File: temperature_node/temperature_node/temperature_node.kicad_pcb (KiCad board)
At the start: 4 copper layers, 21 x 34 mm, 34 parts, among them CN1 UART, J1 USB_C_Receptacle_USB2.0_16P, J2 S2B-PH-K-S, U1 SHT40-AD1B-R3, U2 MCP73831-2-OT, U3 MIC5504-3.3YM5, U4 ESP32-C3-WROOM-02

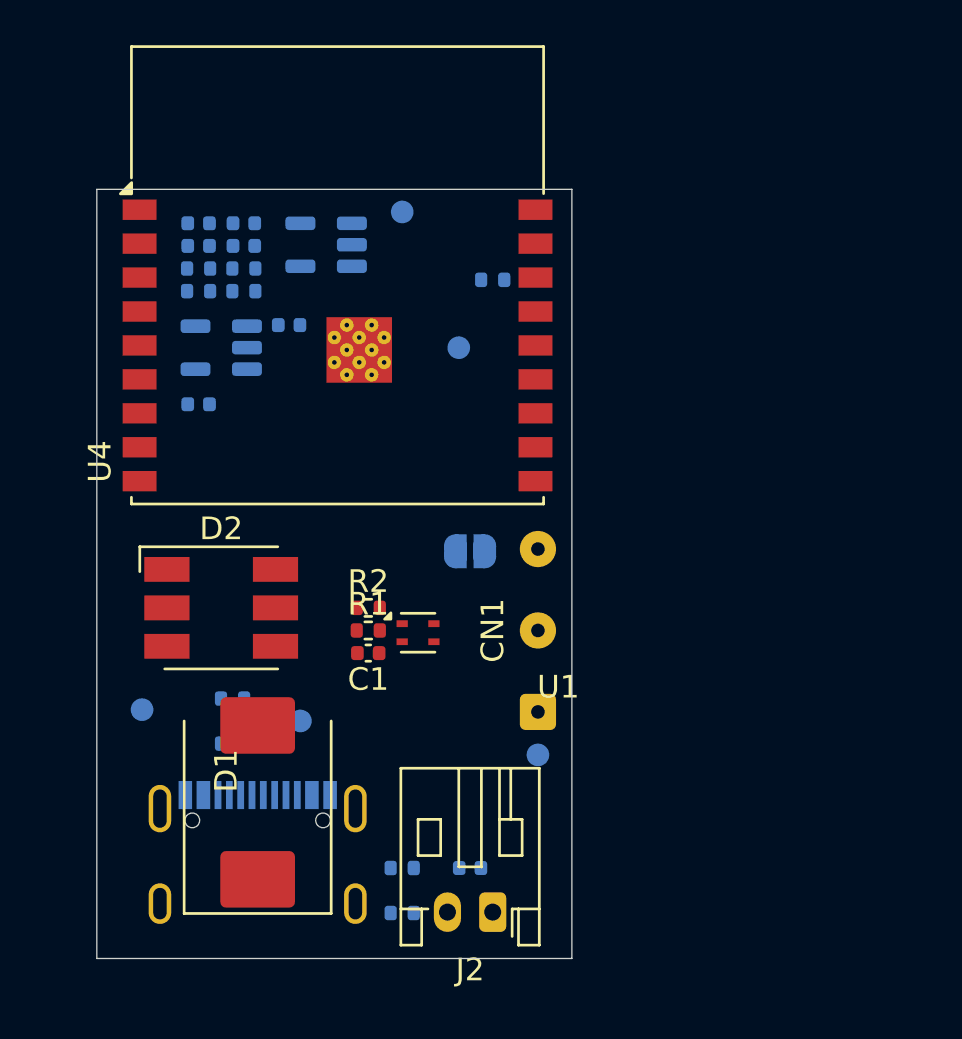
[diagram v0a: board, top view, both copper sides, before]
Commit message: Continue making the board smaller
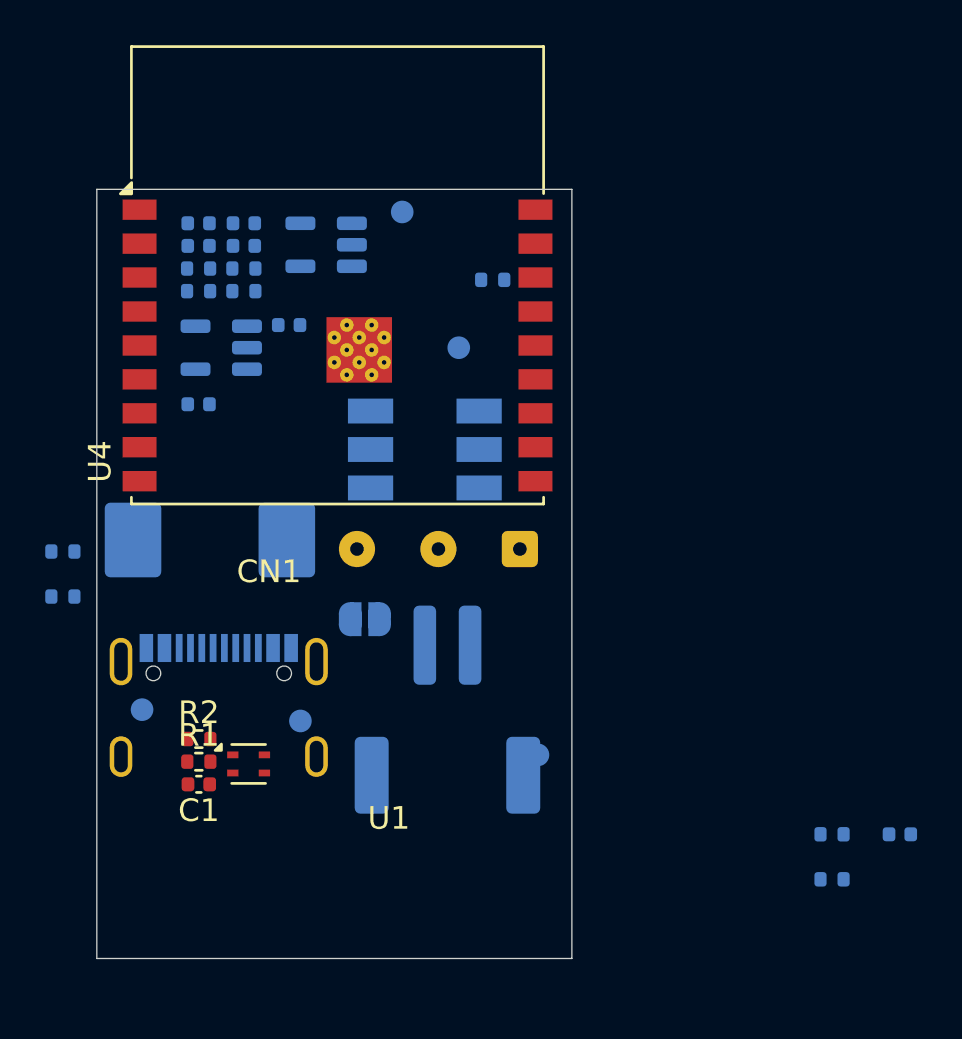
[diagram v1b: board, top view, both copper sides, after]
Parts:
- D1, D2: moved to B.Cu
- J2: footprint Connector_JST:JST_PH_S2B-PH-K_1x02_P2.00mm_Horizontal -> Connector_JST:JST_PH_S2B-PH-SM4-TB_1x02-1MP_P2.00mm_Horizontal; moved to B.Cu
- moved C3 19.1 mm to (157.5, 108.5)
- moved R11 19.1 mm to (154.5, 108.5)
- moved R12 19.1 mm to (154.5, 110.5)
- moved D1 11.8 mm to (127.0, 95.5), turned to 180 degrees
- moved D2 11.4 mm to (136.5, 91.5), turned to 180 degrees
- moved R5 9.92 mm to (120.5, 96.0)
- moved R6 9.92 mm to (120.5, 98.0)
- moved C1 9.47 mm to (126.5, 106.3)
- moved R1 9.47 mm to (126.5, 105.3)
- moved R2 9.47 mm to (126.5, 104.3)
- moved U1 9.47 mm to (128.7, 105.4)
- moved J2 9.17 mm to (137.5, 103.0)
- moved CN1 7.24 mm to (140.7, 95.9), turned to 180 degrees
- moved J1 6.72 mm to (127.4, 104.0)
- moved JP1 5.53 mm to (133.8, 99.0)
